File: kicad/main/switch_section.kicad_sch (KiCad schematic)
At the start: 27 parts, among them SW6 GOAL, SW7 START, SW8 AUX1, U7 AZ1117CH-3.3, U8 PCF8574PW

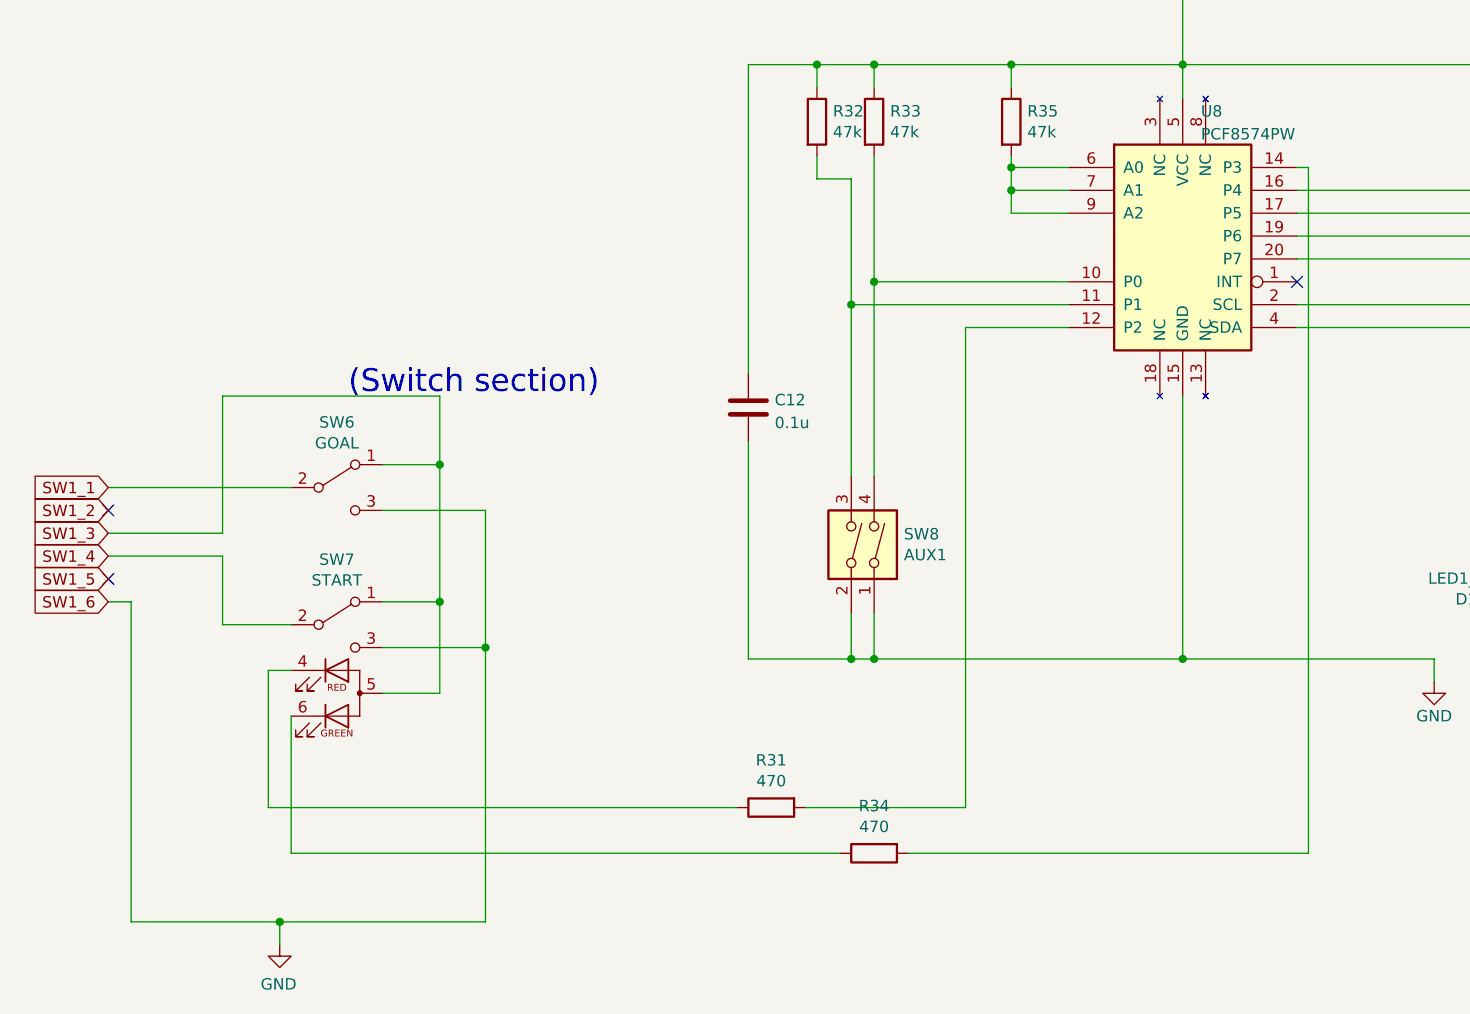
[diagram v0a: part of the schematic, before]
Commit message: SW-LED changed
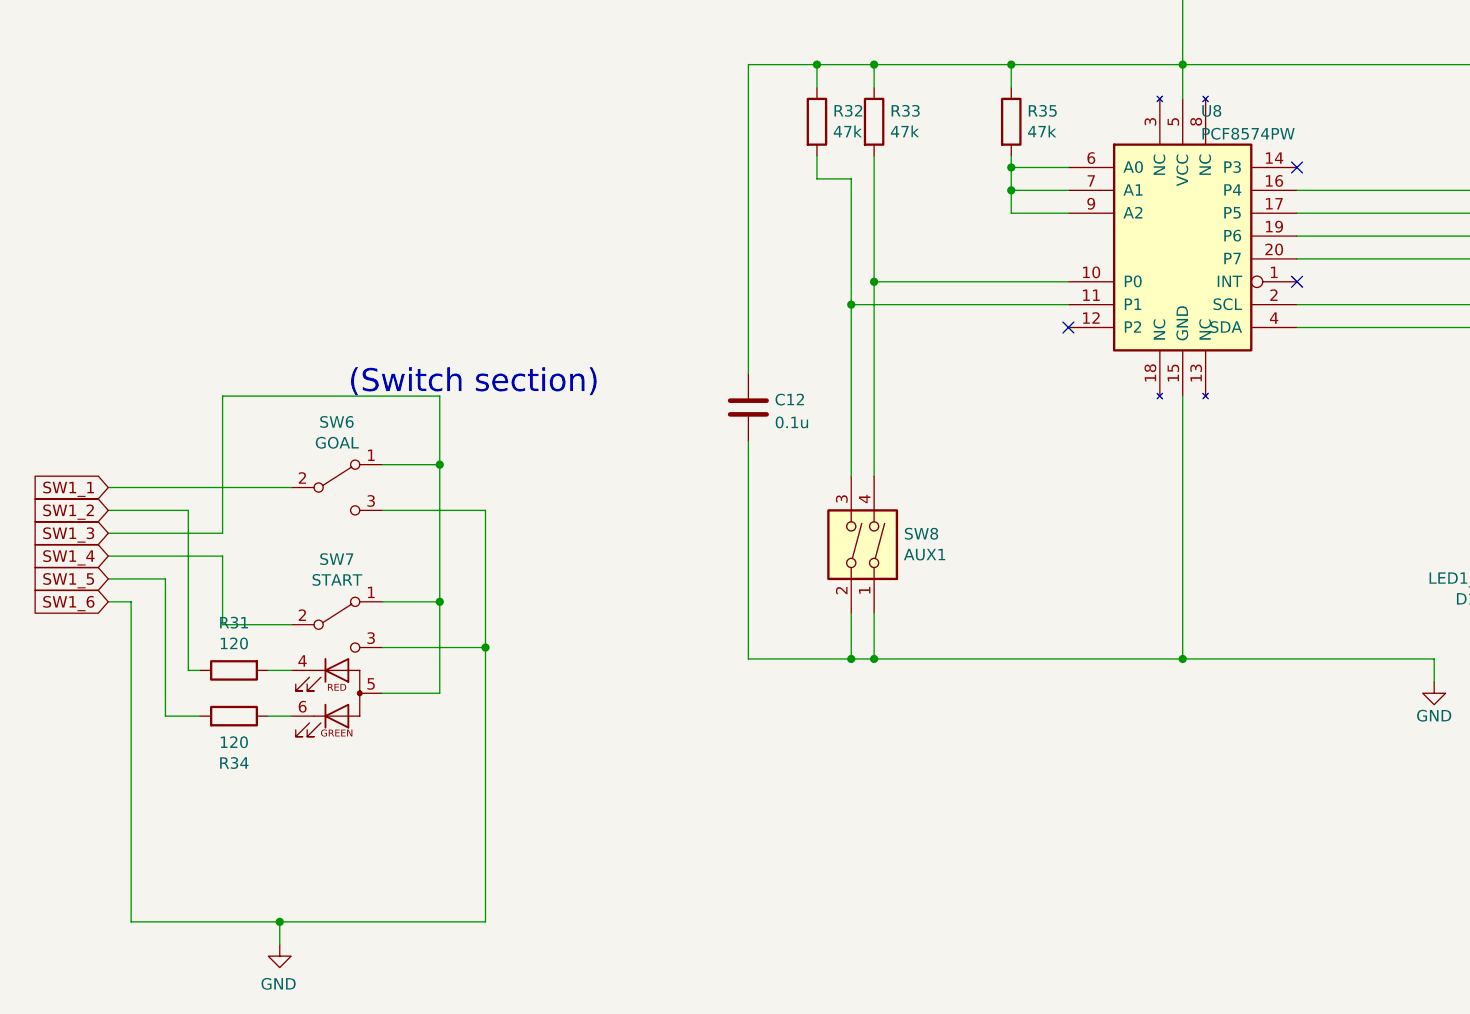
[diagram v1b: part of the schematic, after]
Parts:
- R31, R34: value 470 -> 120
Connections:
- net SW1_2: now also R31.1
- net SW1_5: now also R34.2
- net at SW7.4 (KR): now also R31.2; no longer R31.1
- net at U8.14 (P3): no longer R34.2
- net at U8.12 (P2): no longer R31.2
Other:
- moved on the sheet: R31, R34
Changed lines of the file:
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@@
   )
   (no_connect (at 166.37 113.03))
-  (no_connect (at 34.29 138.43))
-  (no_connect (at 34.29 146.05))
+  (no_connect (at 140.97 118.11))
+  (no_connect (at 166.37 100.33))
   (bus_entry (at 259.08 118.11) (size -2.54 -2.54)
     (stroke (width 0) (type default) (color 0 0 0 0))
@@
     (stroke (width 0) (type default) (color 0 0 0 0))
   )
-  (wire (pts (xy 54.61 161.29) (xy 54.61 176.53))
+  (wire (pts (xy 52.07 161.29) (xy 54.61 161.29))
     (stroke (width 0) (type default) (color 0 0 0 0))
   )
@@
     (stroke (width 0) (type default) (color 0 0 0 0))
   )
+  (wire (pts (xy 34.29 146.05) (xy 40.64 146.05))
+    (stroke (width 0) (type default) (color 0 0 0 0))
+  )
   (wire (pts (xy 105.41 130.81) (xy 105.41 154.94))
     (stroke (width 0) (type default) (color 0 0 0 0))
@@
     (stroke (width 0) (type default) (color 0 0 0 0))
   )
+  (wire (pts (xy 40.64 146.05) (xy 40.64 161.29))
+    (stroke (width 0) (type default) (color 0 0 0 0))
+  )
   (wire (pts (xy 46.99 125.73) (xy 71.12 125.73))
     (stroke (width 0) (type default) (color 0 0 0 0))
@@
     (stroke (width 0) (type default) (color 0 0 0 0))
   )
+  (wire (pts (xy 43.18 156.21) (xy 43.18 138.43))
+    (stroke (width 0) (type default) (color 0 0 0 0))
+  )
   (wire (pts (xy 54.61 151.13) (xy 46.99 151.13))
     (stroke (width 0) (type default) (color 0 0 0 0))
@@
     (stroke (width 0) (type default) (color 0 0 0 0))
   )
-  (wire (pts (xy 111.76 171.45) (xy 129.54 171.45))
-    (stroke (width 0) (type default) (color 0 0 0 0))
-  )
   (wire (pts (xy 71.12 148.59) (xy 71.12 158.75))
     (stroke (width 0) (type default) (color 0 0 0 0))
@@
     (stroke (width 0) (type default) (color 0 0 0 0))
   )
-  (wire (pts (xy 129.54 118.11) (xy 140.97 118.11))
-    (stroke (width 0) (type default) (color 0 0 0 0))
-  )
   (wire (pts (xy 153.67 88.9) (xy 233.68 88.9))
     (stroke (width 0) (type default) (color 0 0 0 0))
@@
     (stroke (width 0) (type default) (color 0 0 0 0))
   )
-  (wire (pts (xy 167.64 100.33) (xy 167.64 176.53))
-    (stroke (width 0) (type default) (color 0 0 0 0))
-  )
   (wire (pts (xy 34.29 140.97) (xy 46.99 140.97))
     (stroke (width 0) (type default) (color 0 0 0 0))
@@
     (stroke (width 0) (type default) (color 0 0 0 0))
   )
-  (wire (pts (xy 123.19 176.53) (xy 167.64 176.53))
-    (stroke (width 0) (type default) (color 0 0 0 0))
-  )
   (wire (pts (xy 46.99 50.8) (xy 54.61 50.8))
     (stroke (width 0) (type default) (color 0 0 0 0))
@@
     (stroke (width 0) (type default) (color 0 0 0 0))
   )
-  (wire (pts (xy 129.54 118.11) (xy 129.54 171.45))
-    (stroke (width 0) (type default) (color 0 0 0 0))
-  )
   (wire (pts (xy 134.62 105.41) (xy 140.97 105.41))
     (stroke (width 0) (type default) (color 0 0 0 0))
   )
-  (wire (pts (xy 52.07 171.45) (xy 104.14 171.45))
-    (stroke (width 0) (type default) (color 0 0 0 0))
-  )
   (wire (pts (xy 64.77 133.35) (xy 71.12 133.35))
     (stroke (width 0) (type default) (color 0 0 0 0))
@@
     (stroke (width 0) (type default) (color 0 0 0 0))
   )
-  (wire (pts (xy 166.37 100.33) (xy 167.64 100.33))
-    (stroke (width 0) (type default) (color 0 0 0 0))
-  )
   (wire (pts (xy 64.77 138.43) (xy 76.2 138.43))
     (stroke (width 0) (type default) (color 0 0 0 0))
@@
     (stroke (width 0) (type default) (color 0 0 0 0))
   )
-  (wire (pts (xy 52.07 156.21) (xy 52.07 171.45))
-    (stroke (width 0) (type default) (color 0 0 0 0))
-  )
   (wire (pts (xy 119.38 113.03) (xy 140.97 113.03))
     (stroke (width 0) (type default) (color 0 0 0 0))
@@
     (stroke (width 0) (type default) (color 0 0 0 0))
   )
-  (wire (pts (xy 54.61 176.53) (xy 115.57 176.53))
+  (wire (pts (xy 40.64 161.29) (xy 44.45 161.29))
     (stroke (width 0) (type default) (color 0 0 0 0))
   )
@@
     (stroke (width 0) (type default) (color 0 0 0 0))
   )
+  (wire (pts (xy 44.45 156.21) (xy 43.18 156.21))
+    (stroke (width 0) (type default) (color 0 0 0 0))
+  )
   (wire (pts (xy 46.99 140.97) (xy 46.99 125.73))
     (stroke (width 0) (type default) (color 0 0 0 0))
@@
   )
   (wire (pts (xy 54.61 135.89) (xy 34.29 135.89))
+    (stroke (width 0) (type default) (color 0 0 0 0))
+  )
+  (wire (pts (xy 34.29 138.43) (xy 43.18 138.43))
     (stroke (width 0) (type default) (color 0 0 0 0))
   )
@@
     (pin "3")
   )
-  (symbol (lib_id "Device:R") (at 119.38 176.53 90) (mirror x) (unit 1)
+  (symbol (lib_id "Device:R") (at 48.26 161.29 270) (mirror x) (unit 1)
     (in_bom yes) (on_board yes)
-    (property "Reference" "R34" (id 0) (at 119.38 171.2722 90))
-    (property "Value" "470" (id 1) (at 119.38 173.5836 90))
-    (property "Footprint" "Resistor_SMD:R_0603_1608Metric_Pad0.98x0.95mm_HandSolder" (id 2) (at 119.38 174.752 90)
-      (effects (font (size 1.27 1.27)) hide)
-    )
-    (property "Datasheet" "~" (id 3) (at 119.38 176.53 0)
+    (property "Reference" "R34" (id 0) (at 48.26 166.5478 90))
+    (property "Value" "120" (id 1) (at 48.26 164.2364 90))
+    (property "Footprint" "Resistor_SMD:R_0603_1608Metric_Pad0.98x0.95mm_HandSolder" (id 2) (at 48.26 163.068 90)
+      (effects (font (size 1.27 1.27)) hide)
+    )
+    (property "Datasheet" "~" (id 3) (at 48.26 161.29 0)
       (effects (font (size 1.27 1.27)) hide)
     )
@@
     (pin "2")
   )
-  (symbol (lib_id "Device:R") (at 107.95 171.45 90) (mirror x) (unit 1)
+  (symbol (lib_id "Device:R") (at 48.26 156.21 90) (mirror x) (unit 1)
     (in_bom yes) (on_board yes)
-    (property "Reference" "R31" (id 0) (at 107.95 166.1922 90))
-    (property "Value" "470" (id 1) (at 107.95 168.5036 90))
-    (property "Footprint" "Resistor_SMD:R_0603_1608Metric_Pad0.98x0.95mm_HandSolder" (id 2) (at 107.95 169.672 90)
-      (effects (font (size 1.27 1.27)) hide)
-    )
-    (property "Datasheet" "~" (id 3) (at 107.95 171.45 0)
-      (effects (font (size 1.27 1.27)) hide)
-    )
+    (property "Reference" "R31" (id 0) (at 48.26 150.9522 90))
+    (property "Value" "120" (id 1) (at 48.26 153.2636 90))
+    (property "Footprint" "Resistor_SMD:R_0603_1608Metric_Pad0.98x0.95mm_HandSolder" (id 2) (at 48.26 154.432 90)
+      (effects (font (size 1.27 1.27)) hide)
+    )
+    (property "Datasheet" "~" (id 3) (at 48.26 156.21 0)
+      (effects (font (size 1.27 1.27)) hide)
+    )
